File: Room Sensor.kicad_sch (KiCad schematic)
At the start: 15 parts, among them SW1 SW_Push, SW2 SW_Push, SW3 SW_Push, SW4 SW_Push, U2 ESP32-C3_SUPERMINI_TH

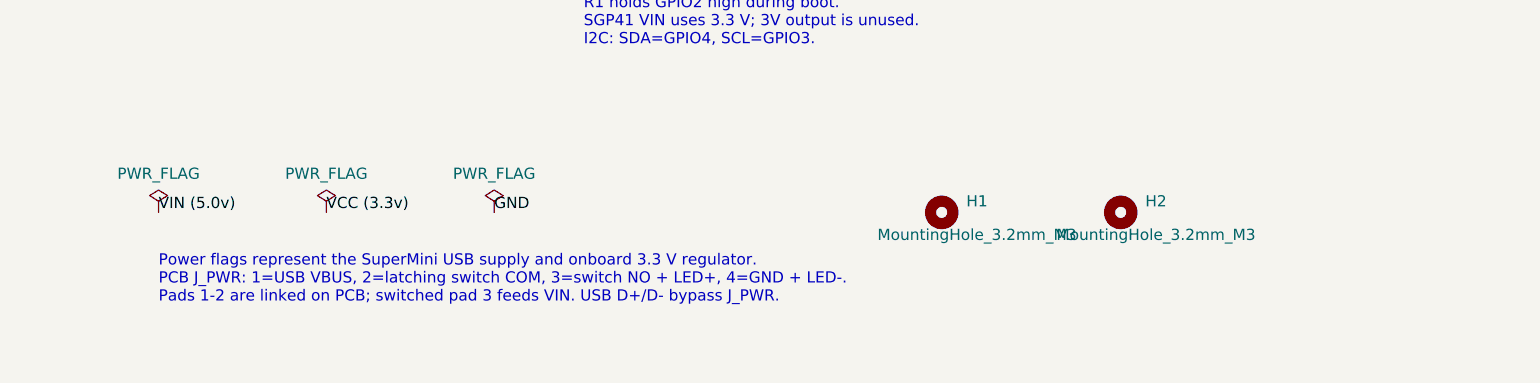
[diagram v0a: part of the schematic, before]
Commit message: Add board-mounted USB-C power input
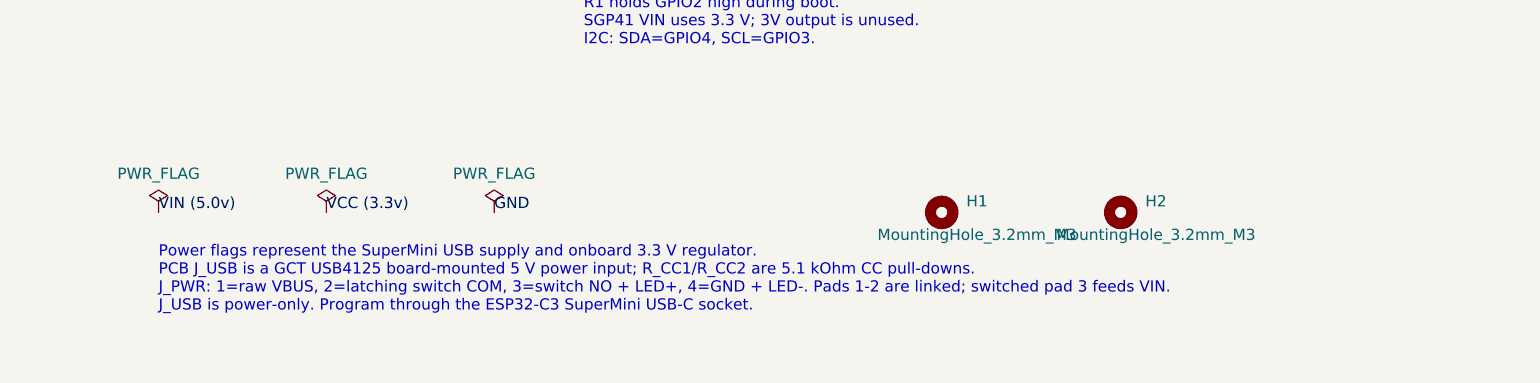
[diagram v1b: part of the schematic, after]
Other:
- note added: "Power flags represent the SuperMini USB supply and onboard 3.3 V regulator. PCB J_USB is a GCT USB4125 board-mounted 5 V power input; R_CC1/R_CC2 are 5.1 kOhm CC pull-downs. J_PWR: 1=raw VBUS, 2=latching switch COM, 3=switch NO + LED+, 4=GND + LED-. Pads 1-2 are linked; switched pad 3 feeds VIN. J_USB is power-only. Program through the ESP32-C3 SuperMini USB-C socket."
- note removed: "Power flags represent the SuperMini USB supply and onboard 3.3 V regulator. PCB J_PWR: 1=USB VBUS, 2=latching switch COM, 3=switch NO + LED+, 4=GND + LED-. Pads 1-2 are linked on PCB; switched pad 3 feeds VIN. USB D+/D- bypass J_PWR."
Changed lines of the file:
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@@
 		)
 	)
-	(text "Power flags represent the SuperMini USB supply and onboard 3.3 V regulator.\nPCB J_PWR: 1=USB VBUS, 2=latching switch COM, 3=switch NO + LED+, 4=GND + LED-.\nPads 1-2 are linked on PCB; switched pad 3 feeds VIN. USB D+/D- bypass J_PWR."
+	(text "Power flags represent the SuperMini USB supply and onboard 3.3 V regulator.\nPCB J_USB is a GCT USB4125 board-mounted 5 V power input; R_CC1/R_CC2 are 5.1 kOhm CC pull-downs.\nJ_PWR: 1=raw VBUS, 2=latching switch COM, 3=switch NO + LED+, 4=GND + LED-. Pads 1-2 are linked; switched pad 3 feeds VIN.\nJ_USB is power-only. Program through the ESP32-C3 SuperMini USB-C socket."
 		(exclude_from_sim no)
 		(at 111.76 161.29 0)
